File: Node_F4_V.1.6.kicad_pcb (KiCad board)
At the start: 2 copper layers, 56 x 100 mm, 171 parts, among them IC2 MP1584EN, J1 Conn_Jack-DC, J2 Conn_02x12_Odd_Even, J3 Micro_SD_Card, J4 RF_IPEX_U.FL-R-SMT, J5 Conn_01x06, J6 Conn_01x06, J7 RS485, J8 LoRa_Anten, Q2 MMBT3904L, Q3 BC847, SW1 SW_Push, SW2 SW_Push, SW3 SW_Push, U1 SX1278, U2 SP3485EN, U3 STM32F407VETx, U4 Flash_W25Q128, U5 DS3231M, U6 ESP32-D0WD-V3, U8 MASWSS0192, Y1 8MHz, Y2 40MHz, Y3 32MHz

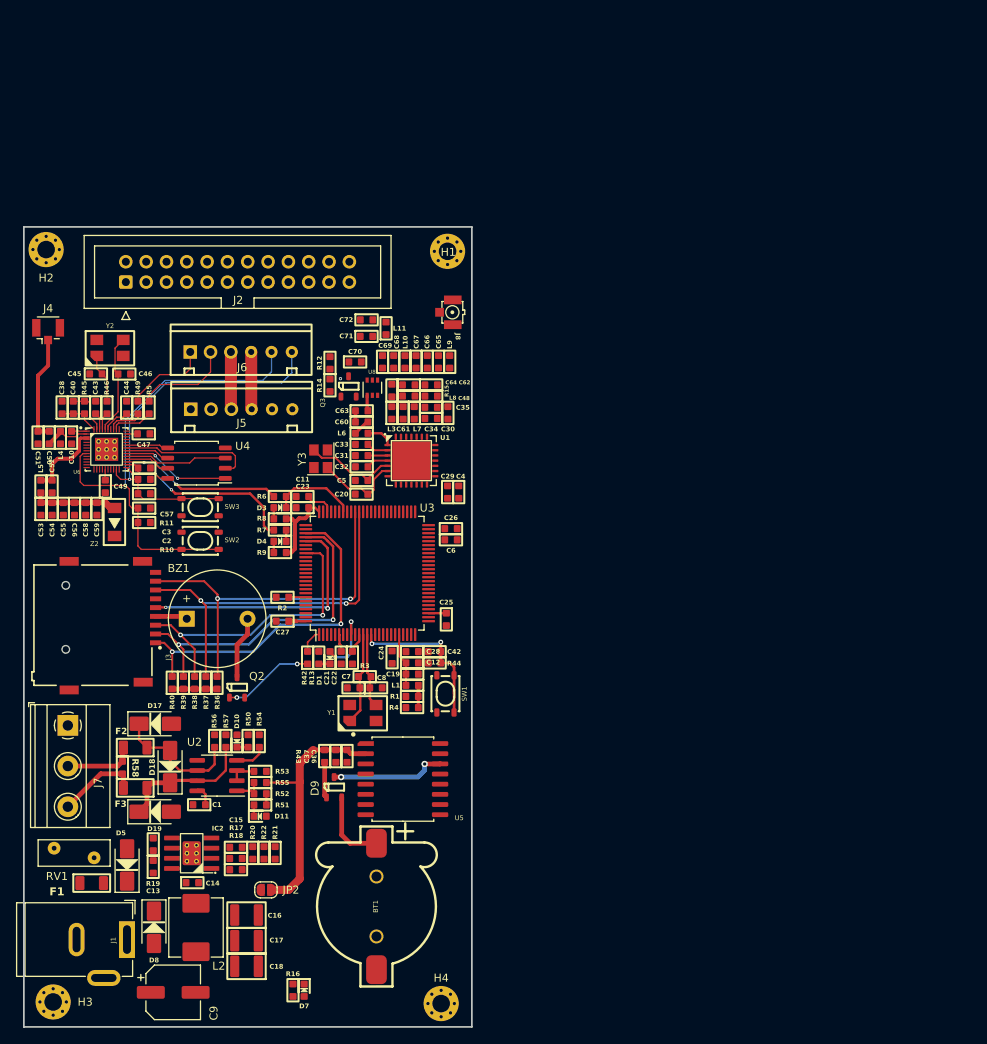
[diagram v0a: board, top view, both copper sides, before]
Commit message: DI track
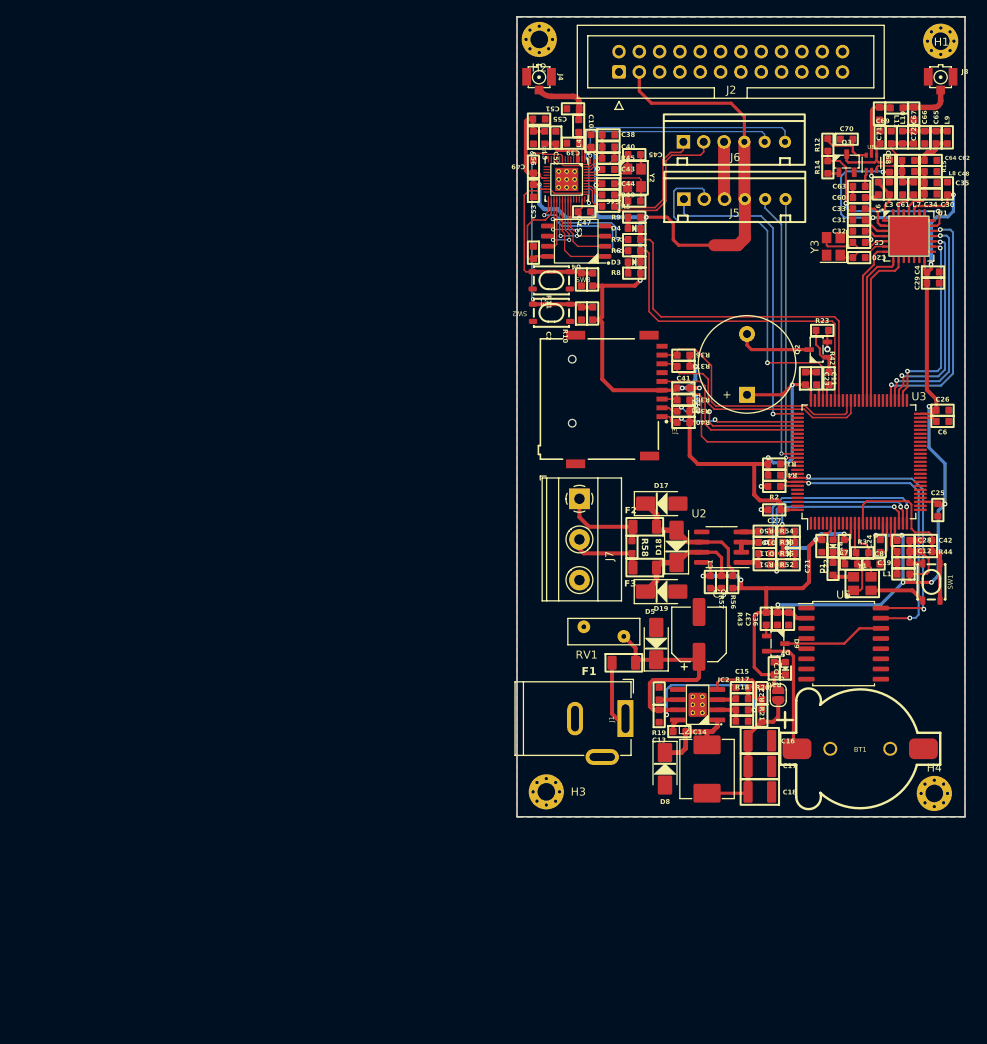
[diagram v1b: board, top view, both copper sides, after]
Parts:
- removed C50: 5.6pF, Anh_Footprints:C_0603
- removed C54: 100nF, Anh_Footprints:C_0603
- removed C58: 10uF, Anh_Footprints:C_0603
- removed C59: 1uF, Anh_Footprints:C_0603
- removed R46: TBD, Anh_Footprints:R_0603
- removed Z2: D_Zener, IVS_FOOTPRINTS:D_MiniMELF
- added C39: NC, Anh_Footprints:C_0603, F.Cu at (124.5, 54.8)
- added C41: 100nF, Anh_Footprints:C_0603, F.Cu at (138.3, 85.4)
- added R23: 10K, Anh_Footprints:R_0603, F.Cu at (155.7, 78.2)
- C51: value 2.4pF -> NC
- C71, C72: value 6.8pF -> NC
- D9, Q2, Q3: footprint IVS_FOOTPRINTS:SOT23-3 -> Anh_Footprints:SOT23-3
- J2: value Conn_02x12_Odd_Even -> IDC_LCD_KEYPAD
- J4: footprint Connector_Coaxial:U.FL_Hirose_U.FL-R-SMT-1_Vertical -> Anh_Footprints:IPEX_Antena_Connector
- J5: value Conn_01x06 -> SWD
- J6: value Conn_01x06 -> WiFi_Prog
- L4: value 2.7nH -> 2.2nH
- U4: footprint Package_SO:SOIC-8_5.23x5.23mm_P1.27mm -> Anh_Footprints:SOIC-8_5.23x5.23
- U5: footprint IVS_FOOTPRINTS:SOIC-16W_7.5x10.3mm_P1.27mm -> Package_SO:SOIC-16W_7.5x10.3mm_P1.27mm
- Y1, Y2: footprint IVS_FOOTPRINTS:Crystal_SMD_5032-4Pin_5.0x3.2mm -> Anh_Footprints:Crystal_3225_4P_1-4
- moved Q2 85.4 mm to (155.2, 80.6)
- moved C9 79.5 mm to (140.2, 116.2), turned to 90 degrees
- moved C51 78.5 mm to (124.5, 50.5), turned to 180 degrees
- moved C55 76.9 mm to (120.2, 51.8), turned to 180 degrees
- moved C52 76.6 mm to (122.3, 54.1), turned to -90 degrees
- moved L5 76.6 mm to (121.0, 54.1), turned to -90 degrees
- moved C38 76.3 mm to (128.9, 53.8), turned to 0 degrees
- moved L4 75.6 mm to (125.2, 52.6)
- moved BZ1 75.4 mm to (146.2, 86.2), turned to 90 degrees
- moved C10 74.8 mm to (126.8, 54.5), turned to 90 degrees
- moved C40 74.4 mm to (128.9, 55.3), turned to 180 degrees
- moved R42 73.9 mm to (156.5, 84.2), turned to -90 degrees
- moved C56 73.8 mm to (119.5, 54.1)
- moved D11 73.8 mm to (151.4, 106.1), turned to 180 degrees
- moved C53 73.3 mm to (119.6, 60.8)
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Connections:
- C45 pad 2: Net-(C45-Pad2) -> Net-(U6-XTAL_P)
- J7 pad 1: GND -> /A+
- J7 pad 2: /A+ -> /B-
- J7 pad 3: /B- -> GND
- L4 pad 1: Net-(U6-LNA_IN) -> Net-(J4-In)
- L4 pad 2: GND -> Net-(U6-LNA_IN)
- U3 pad 1: /BUZZER -> unconnected-(U3-PE2-Pad1)
- U3 pad 7: unconnected-(U3-PC13-Pad7) -> Net-(D1-A)
- U3 pad 71: unconnected-(U3-PA12-Pad71) -> /BUZZER
- U3 pad 72: unconnected-(U3-PA13-Pad72) -> /SWDIO
- U3 pad 76: unconnected-(U3-PA14-Pad76) -> /SWCLK
- U3 pad 9: Net-(D1-A) -> unconnected-(U3-PC15-Pad9)
- Y2 pad 1: Net-(C45-Pad2) -> Net-(U6-XTAL_P)
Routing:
- net +3.3V: track 107.0 -> 404.6 mm, vias 0 -> 28
- net GND: track 7.19 -> 59.0 mm, vias 0 -> 6
- net /SWDIO: track 0.00 -> 48.6 mm, vias 0 -> 1
- net VCC: track 0.00 -> 46.3 mm, vias 0 -> 2
- net /ESP_RX: track 1.55 -> 45.2 mm
- net /I2C_SCL: track 0.00 -> 41.0 mm, vias 0 -> 2
- net /SWCLK: track 0.00 -> 40.0 mm, vias 0 -> 1
- net /I2C_SDA: track 0.00 -> 38.4 mm, vias 0 -> 2
- net /UART_TX_LOG: track 0.00 -> 34.7 mm, vias 0 -> 1
- net /UART_RX_LOG: track 0.00 -> 33.9 mm, vias 0 -> 1
- net /ESP_TX: track 10.8 -> 43.3 mm
- net /LORA NSS: track 0.00 -> 30.7 mm, vias 0 -> 2
- net /SPI_MOSI: track 0.00 -> 28.6 mm, vias 0 -> 2
- net /RS485_RO: track 1.48 -> 28.5 mm, vias 0 -> 2
- net /SPI_MISO: track 0.00 -> 26.6 mm, vias 0 -> 2
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- added copper zone on B.Cu, net GND
- added copper zone on F.Cu, net GND

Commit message: 50%
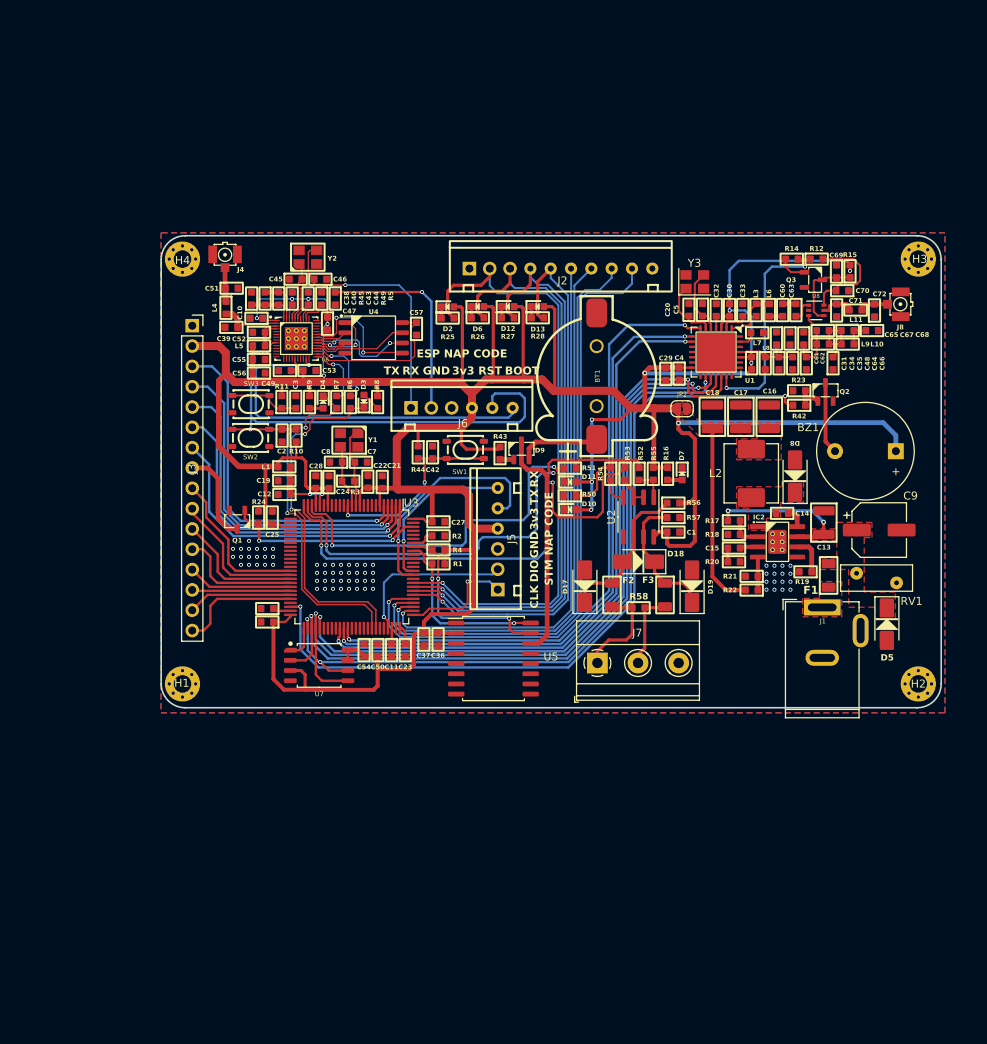
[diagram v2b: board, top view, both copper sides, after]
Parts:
- removed C41: 100nF, Anh_Footprints:C_0603
- removed D1: LED_Blink, Anh_Footprints:LED_0603
- removed R13: 470, Anh_Footprints:R_0603
- removed R36, R37, R38, R39, R40: 10k, Anh_Footprints:R_0603
- added C50: 1u, Anh_Footprints:C_0603, F.Cu at (100.1, 118.2)
- added C54: 100n, Anh_Footprints:C_0603, F.Cu at (98.4, 118.2)
- added D12: LED, Anh_Footprints:LED_0603, F.Cu at (116.4, 75.2)
- added D13: LED, Anh_Footprints:LED_0603, F.Cu at (120.1, 75.2)
- added D2: LED, Anh_Footprints:LED_0603, F.Cu at (108.8, 75.3)
- added D6: LED, Anh_Footprints:LED_0603, F.Cu at (112.6, 75.2)
- added Q1: P_Mosfet, Anh_Footprints:SOT23-3, F.Cu at (82.5, 101.8)
- added R24: 1M, Anh_Footprints:R_0603, F.Cu at (85.2, 101.6)
- added R25: 220, Anh_Footprints:R_0603, F.Cu at (108.8, 76.7)
- added R26: 220, Anh_Footprints:R_0603, F.Cu at (112.6, 76.6)
- added R27: 220, Anh_Footprints:R_0603, F.Cu at (116.4, 76.6)
- added R28: 220, Anh_Footprints:R_0603, F.Cu at (120.1, 76.6)
- added U7: W25Q128JVS, IVS_FOOTPRINTS:SOIC-8_5.23x5.23mm_P1.27mm, F.Cu at (92.8, 120.1)
- C13: footprint Anh_Footprints:C_0603 -> Anh_Footprints:C_1210
- J2: value IDC_LCD_KEYPAD -> Conn_01x10; footprint Connector_IDC:IDC-Header_2x12_P2.54mm_Vertical -> IVS_FOOTPRINTS:XH 2.54 10Pin Female
- J3: value Micro_SD_Card -> Conn_01x16_Female; footprint Anh_Footprints:MicroSD_Socket_9P -> Connector_PinSocket_2.54mm:PinSocket_1x16_P2.54mm_Vertical
- moved H1 124.2 mm to (75.7, 122.4), turned to 180 degrees
- moved H4 115.3 mm to (75.7, 69.3), turned to 180 degrees
- moved H2 93.5 mm to (167.7, 122.4), turned to 180 degrees
- moved C26 88.5 mm to (86.3, 114.7), turned to 180 degrees
- moved C6 87.6 mm to (86.3, 113.0), turned to 180 degrees
- moved C25 83.2 mm to (86.9, 101.6), turned to 90 degrees
- moved H3 81.2 mm to (167.7, 69.3), turned to 180 degrees
- moved L1 78.5 mm to (88.4, 95.3), turned to 0 degrees
- moved C19 78.1 mm to (88.4, 97.0), turned to 0 degrees
- moved C12 77.7 mm to (88.4, 98.7), turned to 180 degrees
- moved C28 73.8 mm to (92.3, 97.1), turned to 90 degrees
- moved C24 69.4 mm to (94.0, 97.2), turned to 90 degrees
- moved C8 68.4 mm to (94.9, 94.7), turned to 180 degrees
- moved Y1 66.6 mm to (96.5, 91.9), turned to 180 degrees
- moved R3 64.9 mm to (96.4, 97.0), turned to 0 degrees
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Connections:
- J2 pad 1: GND -> unconnected-(J2-Pin_1-Pad1)
- J2 pad 2: unconnected-(J2-Pin_2-Pad2) -> /C1
- J2 pad 3: +3.3V -> /C2
- J2 pad 4: unconnected-(J2-Pin_4-Pad4) -> /C3
- J2 pad 5: /TFT_CS -> /C4
- J2 pad 6: unconnected-(J2-Pin_6-Pad6) -> /H1
- J2 pad 7: /TFT_RS -> /H2
- J2 pad 8: unconnected-(J2-Pin_8-Pad8) -> /H3
- J2 pad 9: /TFT_WR -> /H4
- J3 pad 1: /SD_D2 -> GND
- J3 pad 2: /SD_D3 -> +3.3V
- J3 pad 3: /SD_CMD -> /TFT_CS
- J3 pad 4: +3.3V -> /TFT_RS
- J3 pad 5: /SD_CLK -> /TFT_WR
- J3 pad 6: GND -> /TFT_RD
- J3 pad 7: /SD_D0 -> /TFT_RST
- J3 pad 8: /SD_D1 -> Net-(J3-Pin_8)
- J3 pad 9: GND -> /TFT_DB0
- U3 pad 1: unconnected-(U3-PE2-Pad1) -> /TFT_RST
- U3 pad 2: unconnected-(U3-PE3-Pad2) -> /TFT_RD
- U3 pad 3: unconnected-(U3-PE4-Pad3) -> /TFT_WR
- U3 pad 39: unconnected-(U3-PE8-Pad39) -> /TFT_DB0
- U3 pad 4: unconnected-(U3-PE5-Pad4) -> /TFT_RS
- U3 pad 40: unconnected-(U3-PE9-Pad40) -> /TFT_DB1
- U3 pad 41: unconnected-(U3-PE10-Pad41) -> /TFT_DB2
- U3 pad 42: unconnected-(U3-PE11-Pad42) -> /TFT_DB3
- U3 pad 43: unconnected-(U3-PE12-Pad43) -> /TFT_DB4
- U3 pad 44: unconnected-(U3-PE13-Pad44) -> /TFT_DB5
- U3 pad 45: unconnected-(U3-PE14-Pad45) -> /TFT_DB6
- U3 pad 46: unconnected-(U3-PE15-Pad46) -> /TFT_DB7
- U3 pad 48: unconnected-(U3-PB11-Pad48) -> /BUZZER
- U3 pad 5: unconnected-(U3-PE6-Pad5) -> /TFT_CS
- U3 pad 51: unconnected-(U3-PB12-Pad51) -> /W25Q_CS
- U3 pad 65: /SD_D0 -> unconnected-(U3-PC8-Pad65)
- U3 pad 66: /SD_D1 -> unconnected-(U3-PC9-Pad66)
- U3 pad 7: Net-(D1-A) -> unconnected-(U3-PC13-Pad7)
- U3 pad 71: /BUZZER -> unconnected-(U3-PA12-Pad71)
- U3 pad 77: unconnected-(U3-PA15-Pad77) -> /H1
- U3 pad 78: /SD_D2 -> /H2
- U3 pad 79: /SD_D3 -> /H3
- U3 pad 80: /SD_CLK -> /H4
- U3 pad 81: unconnected-(U3-PD0-Pad81) -> /C4
- U3 pad 82: unconnected-(U3-PD1-Pad82) -> /C3
- U3 pad 83: /SD_CMD -> /C2
- U3 pad 84: unconnected-(U3-PD3-Pad84) -> /C1
- U3 pad 98: unconnected-(U3-PE1-Pad98) -> /TFT_LED
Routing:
- net /BUZZER: track 2.09 -> 97.8 mm, vias 0 -> 2
- net +3.3V: track 404.6 -> 497.1 mm, vias 28 -> 13
- net /H4: track 0.00 -> 80.4 mm, vias 0 -> 1
- net /C1: track 0.00 -> 78.4 mm, vias 0 -> 1
- net /H3: track 0.00 -> 76.7 mm, vias 0 -> 1
- net /C2: track 0.00 -> 75.7 mm, vias 0 -> 1
- net /C3: track 0.00 -> 72.8 mm, vias 0 -> 1
- net /H2: track 0.00 -> 70.9 mm, vias 0 -> 1
- net /C4: track 0.00 -> 70.8 mm, vias 0 -> 1
- net /SPI_MOSI: track 28.6 -> 96.7 mm
- net /H1: track 0.00 -> 67.5 mm, vias 0 -> 1
- net /SPI_SCK: track 24.3 -> 89.4 mm, vias 2 -> 3
- net /SPI_MISO: track 26.6 -> 91.2 mm
- net /LORA_RST: track 20.3 -> 80.0 mm, vias 0 -> 2
- net GND: track 59.0 -> 0.00 mm, vias 6 -> 66
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- added copper zone on F.Cu, net Net-(D8-K)
- added copper zone on F.Cu, net Net-(F1-Pad1)
- added copper zone on F.Cu, net Net-(JP2-A)
- added copper zone on F.Cu, net VCC
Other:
- board size 56 x 100 mm -> 97.5 x 59 mm
- board text added: "3v3"
- board text added: "BOOT"
- board text added: "CLK"
- board text added: "DIO"
- board text added: "ESP NAP CODE"
- board text added: "GND"
- board text added: "RST"
- board text added: "RX"
- board text added: "STM NAP CODE"
- board text added: "TX"

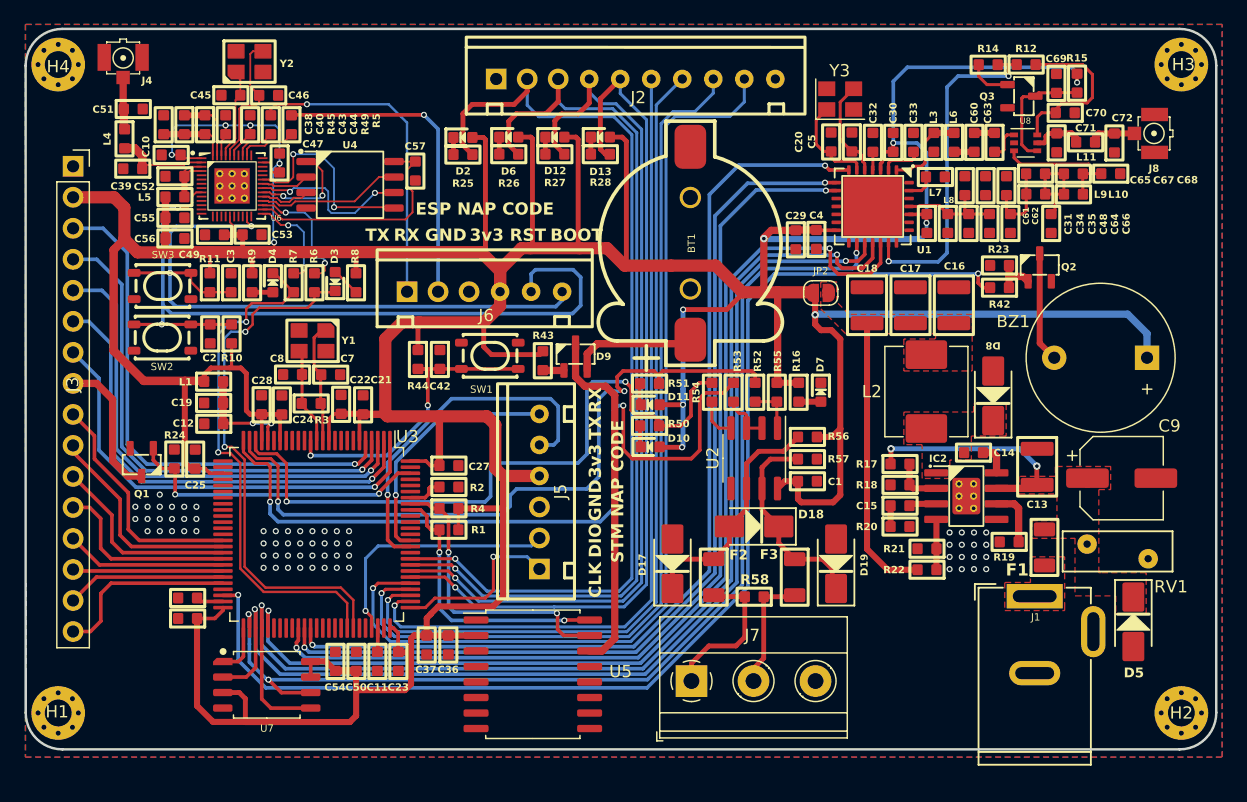
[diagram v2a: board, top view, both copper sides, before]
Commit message: Xep linh kien
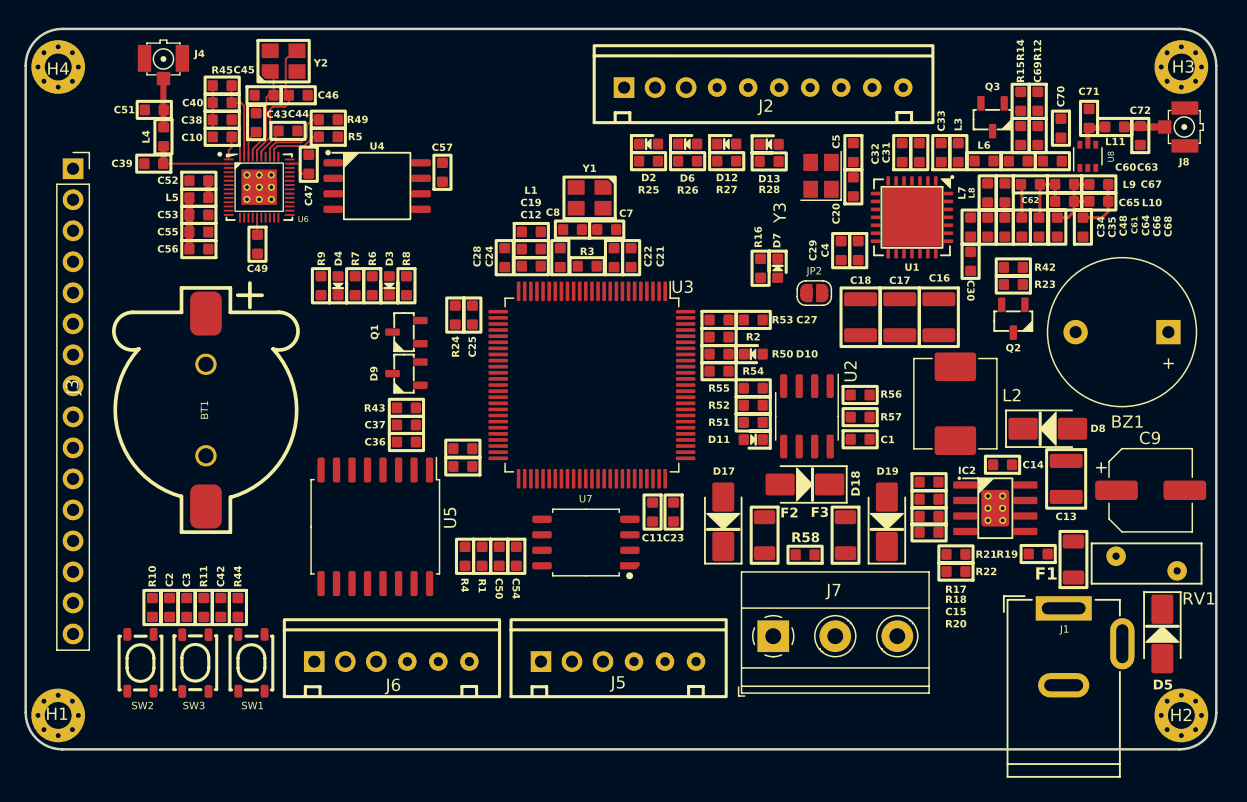
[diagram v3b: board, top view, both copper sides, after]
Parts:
- moved BT1 42.0 mm to (87.8, 97.6), turned to 90 degrees
- moved SW1 31.9 mm to (91.6, 118.3), turned to -90 degrees
- moved J6 31.2 mm to (99.2, 118.2)
- moved SW3 31.1 mm to (86.8, 118.3), turned to 90 degrees
- moved C12 29.0 mm to (114.4, 85.8)
- moved C19 28.9 mm to (114.4, 84.4)
- moved L1 28.8 mm to (114.4, 83.0)
- moved U7 28.6 mm to (118.9, 108.4), turned to 180 degrees
- moved C42 27.1 mm to (89.0, 113.8)
- moved C3 26.8 mm to (86.2, 113.8)
- moved SW2 26.6 mm to (82.5, 118.3), turned to -90 degrees
- moved R11 26.6 mm to (87.6, 113.8)
- moved R24 25.9 mm to (108.2, 89.8)
- moved C8 25.8 mm to (117.8, 82.8)
- moved C24 25.8 mm to (116.8, 85.1)
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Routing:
- net +3.3V: track 497.1 -> 14.7 mm, vias 13 -> 0
- net /BUZZER: track 97.8 -> 0.00 mm, vias 2 -> 0
- net /SPI_MOSI: track 96.7 -> 0.00 mm, vias 2 -> 0
- net /SPI_MISO: track 91.2 -> 0.00 mm, vias 2 -> 0
- net /SPI_SCK: track 89.4 -> 0.00 mm, vias 3 -> 0
- net /LORA NSS: track 86.8 -> 0.00 mm, vias 2 -> 0
- net /H4: track 80.4 -> 0.00 mm, vias 1 -> 0
- net /LORA_RST: track 80.0 -> 0.00 mm, vias 2 -> 0
- net /LORA_DIO1: track 78.9 -> 0.00 mm, vias 2 -> 0
- net /C1: track 78.4 -> 0.00 mm, vias 1 -> 0
- net /LORA_DIO0: track 78.4 -> 0.00 mm, vias 2 -> 0
- net /H3: track 76.7 -> 0.00 mm, vias 1 -> 0
- net /C2: track 75.7 -> 0.00 mm, vias 1 -> 0
- net /C3: track 72.8 -> 0.00 mm, vias 1 -> 0
- net /H2: track 70.9 -> 0.00 mm, vias 1 -> 0
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- removed copper zone on B.Cu, net GND
- removed copper zone on F.Cu, net GND
- removed copper zone on F.Cu, net Net-(D8-K)
- removed copper zone on F.Cu, net Net-(F1-Pad1)
- removed copper zone on F.Cu, net Net-(JP2-A)
- removed copper zone on F.Cu, net VCC
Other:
- board text removed: "3v3"
- board text removed: "BOOT"
- board text removed: "CLK"
- board text removed: "DIO"
- board text removed: "ESP NAP CODE"
- board text removed: "GND"
- board text removed: "RST"
- board text removed: "RX"
- board text removed: "STM NAP CODE"
- board text removed: "TX"
